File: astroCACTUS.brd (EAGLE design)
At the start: 21 parts, among them U1 ATTINY85-20P

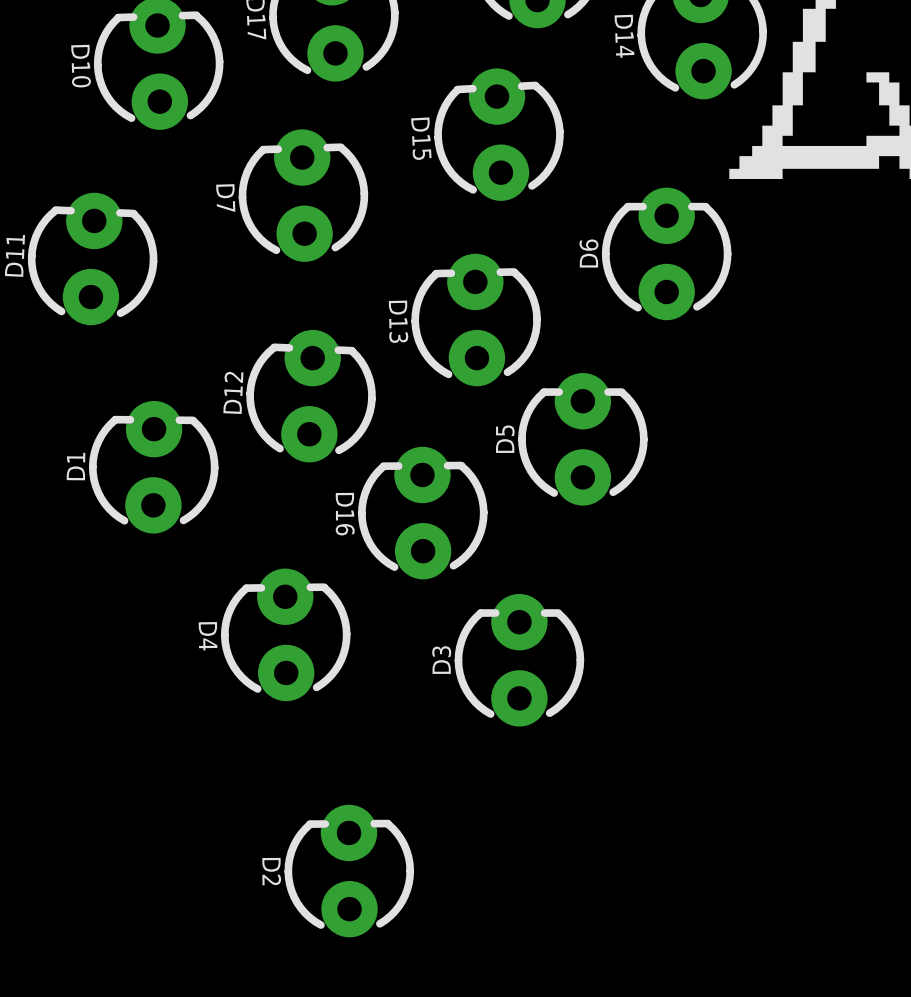
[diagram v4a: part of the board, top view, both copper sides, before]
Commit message: astro boy
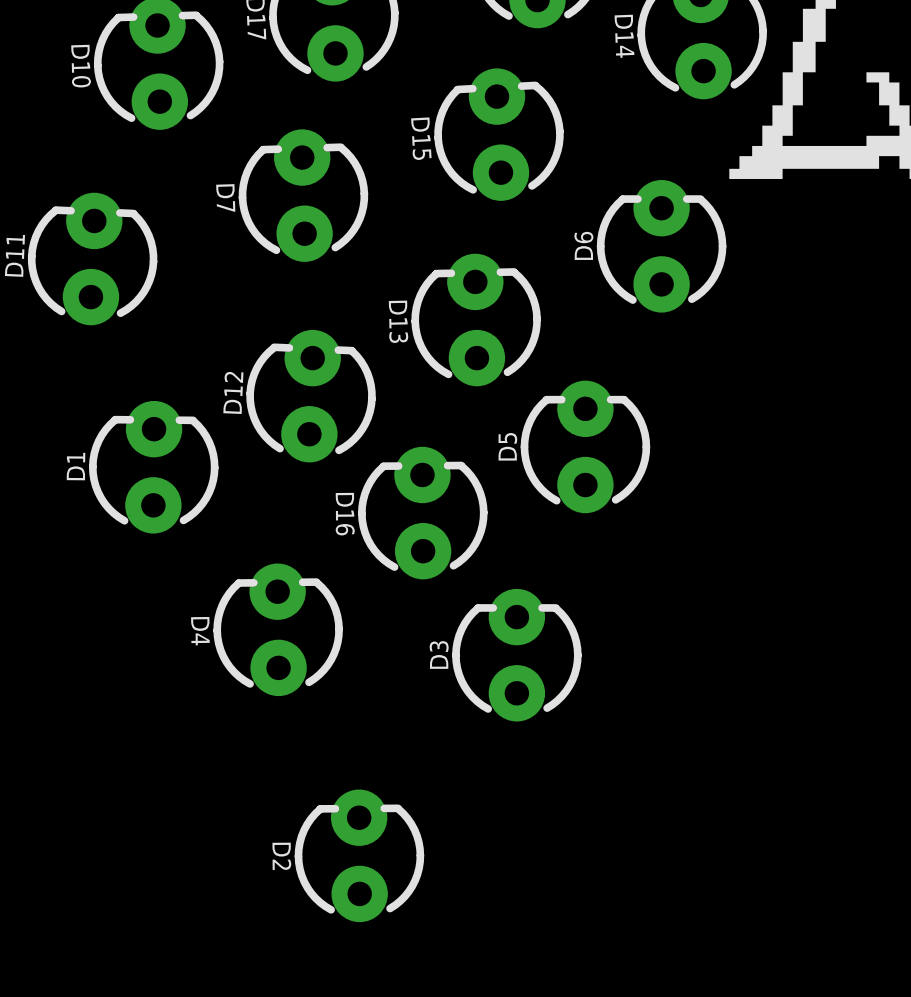
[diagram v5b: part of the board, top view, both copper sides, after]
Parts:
- moved D2 0.61 mm to (23.3, -18.0)
- moved D4 0.31 mm to (20.6, -10.5)
- moved D6 0.31 mm to (33.3, 2.29)
- moved D5 0.27 mm to (30.8, -4.40)
- moved D3 0.19 mm to (28.5, -11.3)
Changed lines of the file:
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@@
 <attribute name="PROD_ID" value="DIO-08794" x="16.41785" y="-5.0791125" size="1.778" layer="27" rot="R89.5" display="off"/>
 </element>
-<element name="D2" library="SparkFun-LED" library_urn="urn:adsk.eagle:library:529" package="LED_3MM" package3d_urn="urn:adsk.eagle:package:39361/1" value="" x="22.936025" y="-18.539765625" rot="R90.4">
-<attribute name="PROD_ID" value="DIO-08794" x="22.936025" y="-18.539765625" size="1.778" layer="27" rot="R90.4" display="off"/>
+<element name="D2" library="SparkFun-LED" library_urn="urn:adsk.eagle:library:529" package="LED_3MM" package3d_urn="urn:adsk.eagle:package:39361/1" value="" x="23.274659375" y="-18.03181875" rot="R90.4">
+<attribute name="PROD_ID" value="DIO-08794" x="23.274659375" y="-18.03181875" size="1.778" layer="27" rot="R90.4" display="off"/>
 </element>
-<element name="D3" library="SparkFun-LED" library_urn="urn:adsk.eagle:library:529" package="LED_3MM" package3d_urn="urn:adsk.eagle:package:39361/1" value="" x="28.607609375" y="-11.513140625" rot="R90">
-<attribute name="PROD_ID" value="DIO-08794" x="28.607609375" y="-11.513140625" size="1.778" layer="27" rot="R90" display="off"/>
+<element name="D3" library="SparkFun-LED" library_urn="urn:adsk.eagle:library:529" package="LED_3MM" package3d_urn="urn:adsk.eagle:package:39361/1" value="" x="28.522953125" y="-11.343821875" rot="R90">
+<attribute name="PROD_ID" value="DIO-08794" x="28.522953125" y="-11.343821875" size="1.778" layer="27" rot="R90" display="off"/>
 </element>
-<element name="D4" library="SparkFun-LED" library_urn="urn:adsk.eagle:library:529" package="LED_3MM" package3d_urn="urn:adsk.eagle:package:39361/1" value="" x="20.81855" y="-10.66655" rot="R90.7">
-<attribute name="PROD_ID" value="DIO-08794" x="20.81855" y="-10.66655" size="1.778" layer="27" rot="R90.7" display="off"/>
+<element name="D4" library="SparkFun-LED" library_urn="urn:adsk.eagle:library:529" package="LED_3MM" package3d_urn="urn:adsk.eagle:package:39361/1" value="" x="20.564575" y="-10.497234375" rot="R90.7">
+<attribute name="PROD_ID" value="DIO-08794" x="20.564575" y="-10.497234375" size="1.778" layer="27" rot="R90.7" display="off"/>
 </element>
-<element name="D5" library="SparkFun-LED" library_urn="urn:adsk.eagle:library:529" package="LED_3MM" package3d_urn="urn:adsk.eagle:package:39361/1" value="" x="30.72305625" y="-4.14786875" rot="R90">
-<attribute name="PROD_ID" value="DIO-08794" x="30.72305625" y="-4.14786875" size="1.778" layer="27" rot="R90" display="off"/>
+<element name="D5" library="SparkFun-LED" library_urn="urn:adsk.eagle:library:529" package="LED_3MM" package3d_urn="urn:adsk.eagle:package:39361/1" value="" x="30.807715625" y="-4.40184375" rot="R90">
+<attribute name="PROD_ID" value="DIO-08794" x="30.807715625" y="-4.40184375" size="1.778" layer="27" rot="R90" display="off"/>
 </element>
-<element name="D6" library="SparkFun-LED" library_urn="urn:adsk.eagle:library:529" package="LED_3MM" package3d_urn="urn:adsk.eagle:package:39361/1" value="" x="33.51626875" y="2.03218125" rot="R90">
-<attribute name="PROD_ID" value="DIO-08794" x="33.51626875" y="2.03218125" size="1.778" layer="27" rot="R90" display="off"/>
+<element name="D6" library="SparkFun-LED" library_urn="urn:adsk.eagle:library:529" package="LED_3MM" package3d_urn="urn:adsk.eagle:package:39361/1" value="" x="33.346953125" y="2.286153125" rot="R90">
+<attribute name="PROD_ID" value="DIO-08794" x="33.346953125" y="2.286153125" size="1.778" layer="27" rot="R90" display="off"/>
 </element>
 <element name="D11" library="SparkFun-LED" library_urn="urn:adsk.eagle:library:529" package="LED_3MM" package3d_urn="urn:adsk.eagle:package:39361/1" value="" x="14.3814875" y="1.862096875" rot="R87.5">
@@
 <wire x1="21.448003125" y1="2.705375" x2="22.477190625" y2="8.715321875" width="0" layer="19" extent="1-1"/>
 <wire x1="14.326090625" y1="0.59330625" x2="21.448003125" y2="2.705375" width="0" layer="19" extent="1-1"/>
-<wire x1="33.51626875" y1="0.76218125" x2="14.326090625" y2="0.59330625" width="0" layer="19" extent="1-1"/>
-<wire x1="30.72305625" y1="-5.41786875" x2="33.51626875" y2="0.76218125" width="0" layer="19" extent="1-1"/>
-<wire x1="20.8340625" y1="-11.936453125" x2="30.72305625" y2="-5.41786875" width="0" layer="19" extent="1-1"/>
-<wire x1="28.607609375" y1="-12.783140625" x2="20.8340625" y2="-11.936453125" width="0" layer="19" extent="1-1"/>
-<wire x1="22.944890625" y1="-19.809734375" x2="28.607609375" y2="-12.783140625" width="0" layer="19" extent="1-1"/>
-<wire x1="16.406765625" y1="-6.3490625" x2="22.944890625" y2="-19.809734375" width="0" layer="19" extent="1-1"/>
+<wire x1="33.346953125" y1="1.016153125" x2="14.326090625" y2="0.59330625" width="0" layer="19" extent="1-1"/>
+<wire x1="30.807715625" y1="-5.67184375" x2="33.346953125" y2="1.016153125" width="0" layer="19" extent="1-1"/>
+<wire x1="20.5800875" y1="-11.7671375" x2="30.807715625" y2="-5.67184375" width="0" layer="19" extent="1-1"/>
+<wire x1="28.522953125" y1="-12.613821875" x2="20.5800875" y2="-11.7671375" width="0" layer="19" extent="1-1"/>
+<wire x1="23.283525" y1="-19.3017875" x2="28.522953125" y2="-12.613821875" width="0" layer="19" extent="1-1"/>
+<wire x1="16.406765625" y1="-6.3490625" x2="23.283525" y2="-19.3017875" width="0" layer="19" extent="1-1"/>
 <wire x1="-53.34" y1="10.16" x2="16.406765625" y2="-6.3490625" width="0" layer="19" extent="1-1"/>
 <wire x1="-44.45" y1="48.26" x2="-53.34" y2="10.16" width="0" layer="19" extent="1-1"/>
@@
 <contactref element="D5" pad="K"/>
 <contactref element="D6" pad="K"/>
-<wire x1="30.72305625" y1="-2.87786875" x2="33.51626875" y2="3.30218125" width="0" layer="19" extent="1-1"/>
-<wire x1="20.803034375" y1="-9.39664375" x2="30.72305625" y2="-2.87786875" width="0" layer="19" extent="1-1"/>
-<wire x1="28.607609375" y1="-10.243140625" x2="20.803034375" y2="-9.39664375" width="0" layer="19" extent="1-1"/>
-<wire x1="22.92715625" y1="-17.26979375" x2="28.607609375" y2="-10.243140625" width="0" layer="19" extent="1-1"/>
-<wire x1="16.42893125" y1="-3.809159375" x2="22.92715625" y2="-17.26979375" width="0" layer="19" extent="1-1"/>
+<wire x1="30.807715625" y1="-3.13184375" x2="33.346953125" y2="3.556153125" width="0" layer="19" extent="1-1"/>
+<wire x1="20.549059375" y1="-9.227328125" x2="30.807715625" y2="-3.13184375" width="0" layer="19" extent="1-1"/>
+<wire x1="28.522953125" y1="-10.073821875" x2="20.549059375" y2="-9.227328125" width="0" layer="19" extent="1-1"/>
+<wire x1="23.265790625" y1="-16.761846875" x2="28.522953125" y2="-10.073821875" width="0" layer="19" extent="1-1"/>
+<wire x1="16.42893125" y1="-3.809159375" x2="23.265790625" y2="-16.761846875" width="0" layer="19" extent="1-1"/>
 <wire x1="-50.8" y1="2.54" x2="16.42893125" y2="-3.809159375" width="0" layer="19" extent="1-1"/>
 </signal>

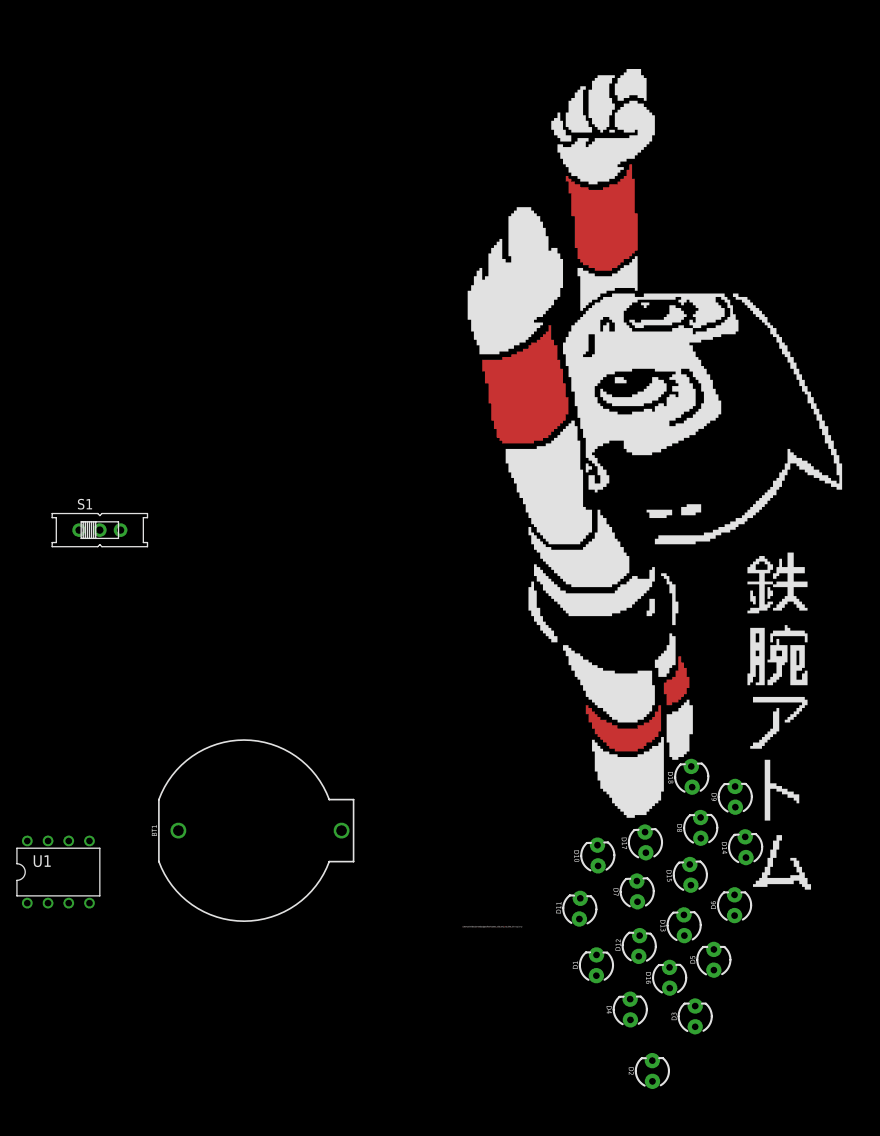
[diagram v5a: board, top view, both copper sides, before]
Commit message: astro boy
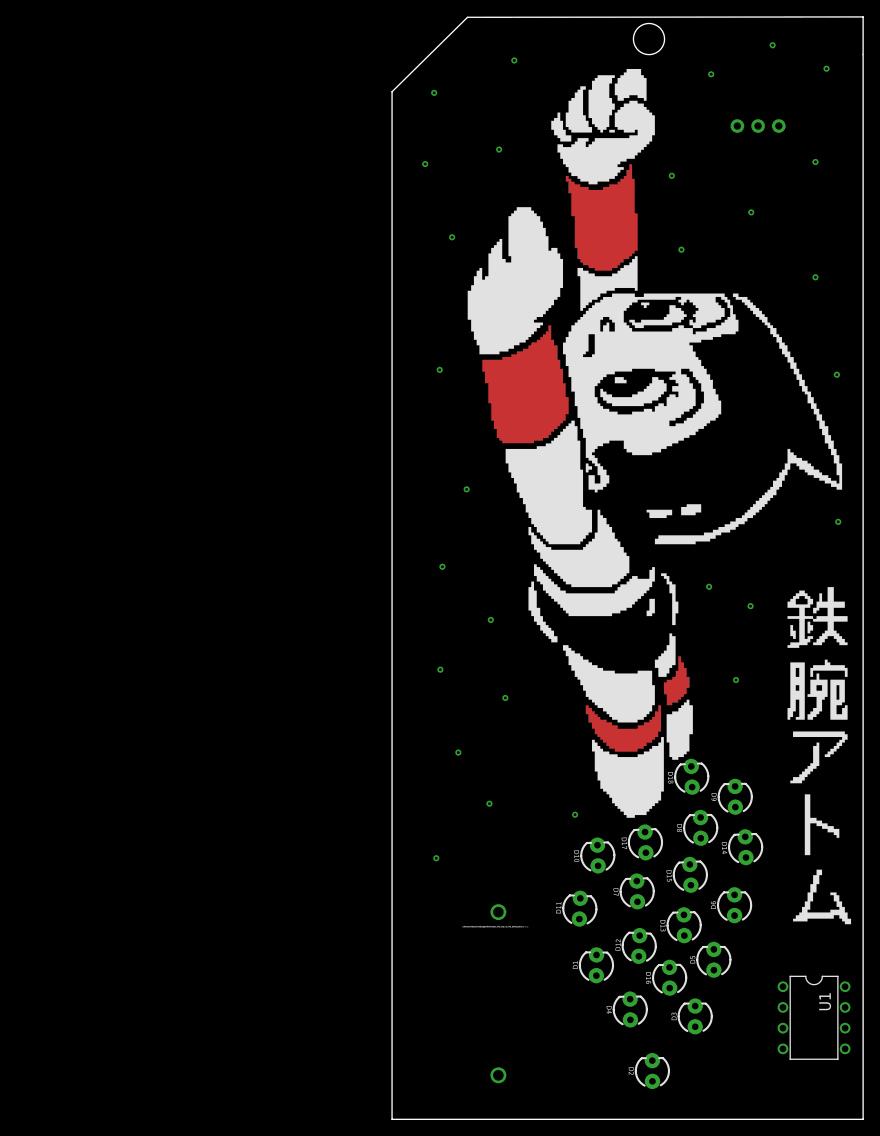
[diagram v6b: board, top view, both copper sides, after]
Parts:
- moved S1 94.7 mm to (36.2, 97.8), flipped to the bottom, turned to 180 degrees
- moved U1 94.3 mm to (43.1, -11.5), turned to 270 degrees
- moved BT1 38.0 mm to (4.40, -10.4), flipped to the bottom, turned to 90 degrees
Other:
- board outline added: 57.7 x 135.1 mm
- board text added: "/Users/chrisbuckner/badges/fresh/astro_silk_only_no_fire_words_bitmap.bmp"

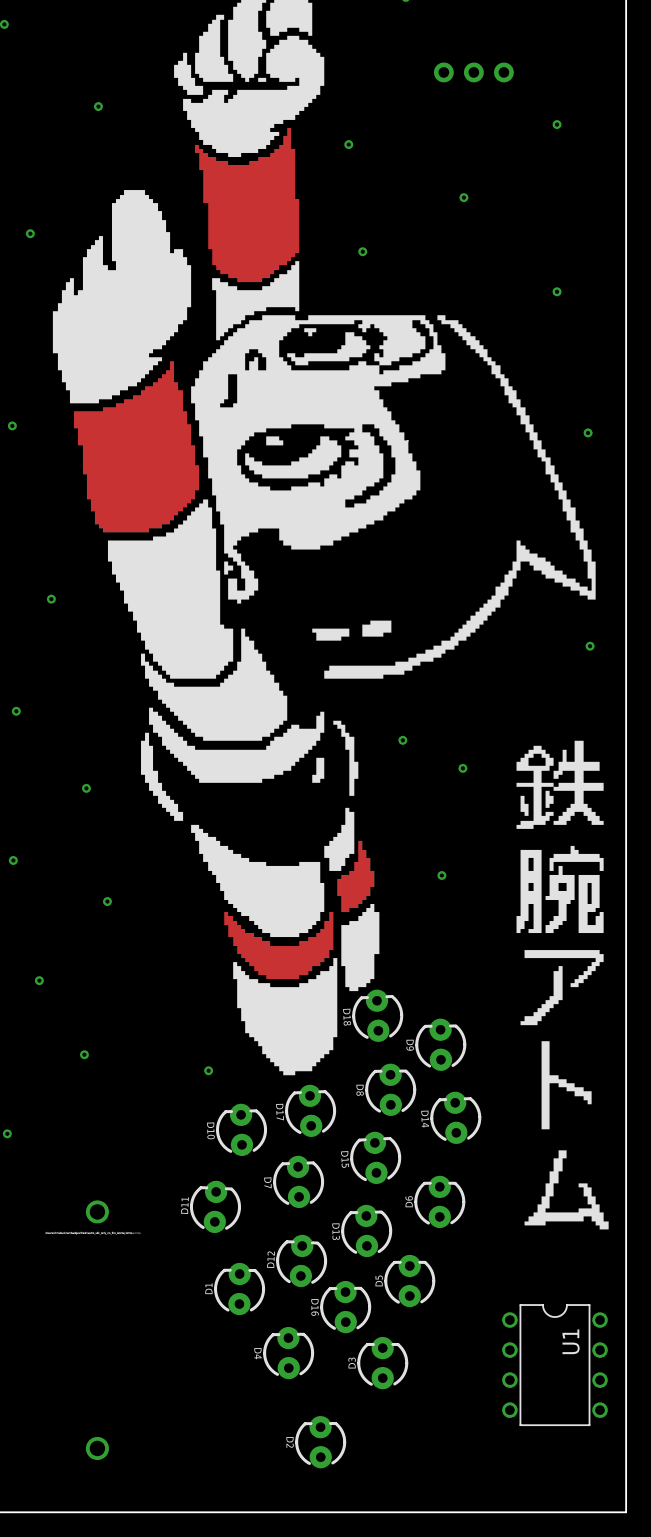
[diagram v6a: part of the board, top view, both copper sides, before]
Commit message: astro boy
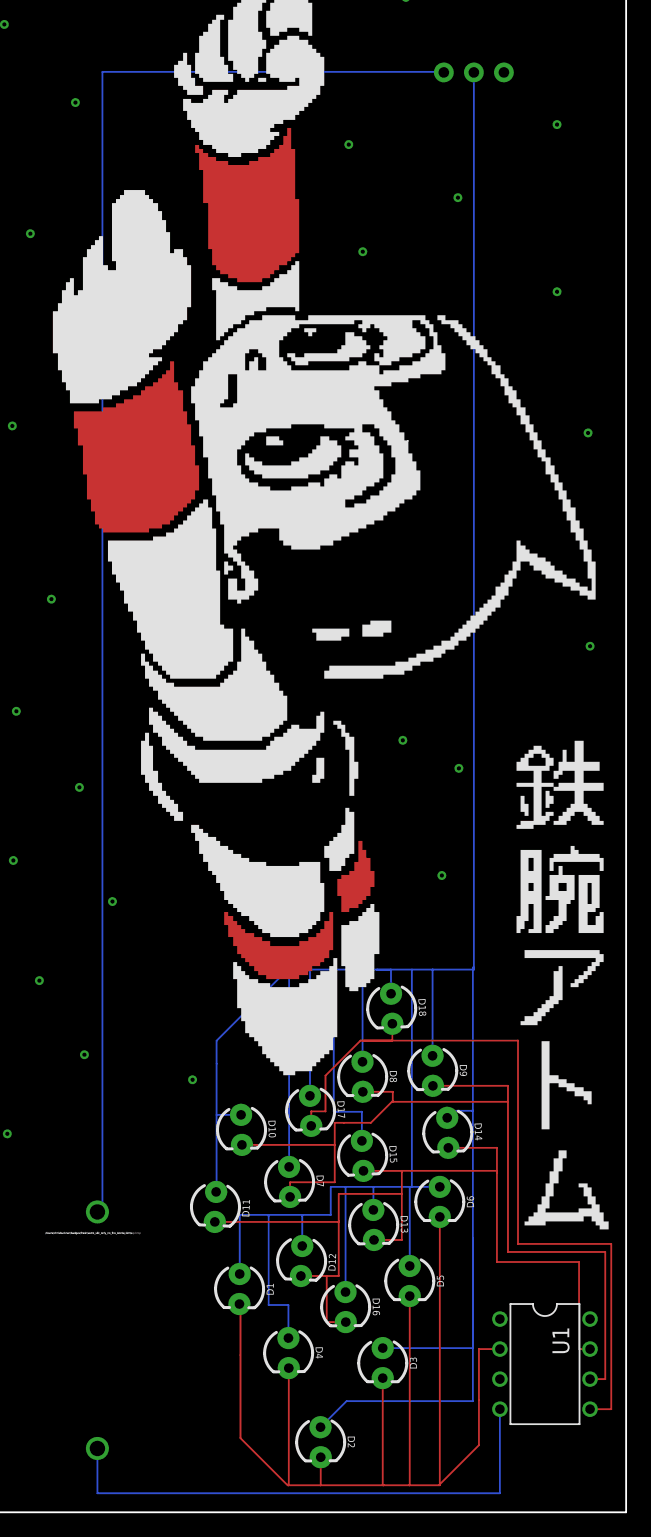
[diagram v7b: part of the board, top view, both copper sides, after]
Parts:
- moved D8 2.61 mm to (26.8, 12.9), turned to 270.6 degrees
- moved D9 2.30 mm to (32.8, 13.4), turned to 270.7 degrees
- moved D14 1.44 mm to (34.0, 8.12), turned to 272.1 degrees
- moved D18 1.33 mm to (29.3, 18.6), turned to 272.5 degrees
- moved D15 1.11 mm to (26.8, 6.18), turned to 273 degrees
- moved U1 0.85 mm to (42.2, -11.4)
- moved D13 0.78 mm to (27.8, 0.34), turned to 271.2 degrees
- moved D7 0.76 mm to (20.6, 3.97), turned to 271.8 degrees
- turned D1 to 269.5 degrees
- turned D10 to 271.7 degrees
- turned D11 to 267.5 degrees
- turned D12 to 267.5 degrees
- turned D16 to 270.5 degrees
- turned D17 to 272.4 degrees
- turned D2 to 270.4 degrees
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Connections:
- net N$31: now also D10.A, D12.A, D13.A, D14.A, D15.A, D16.A, D18.A, D8.A, D9.A
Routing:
- net N$31: track 0.00 -> 323.1 mm
- net N$2: track 0.00 -> 125.5 mm
- net N$1: track 0.00 -> 104.9 mm
- net N$3: track 0.00 -> 80.3 mm
- net N$4: track 0.00 -> 77.4 mm
- net N$6: track 0.00 -> 67.7 mm
- net N$5: track 0.00 -> 44.9 mm
